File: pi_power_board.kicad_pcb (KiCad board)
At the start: 2 copper layers, 34.8 x 23.1 mm, 26 parts, among them J1 381camcon, J2 Conn_02x04_Odd_Even, Q1 SSM3K335R, Q2 SSM3K335R, Q3 DMG2305UX-7, U1 LM74610, U2 TPS2400, U3 DMMT5401

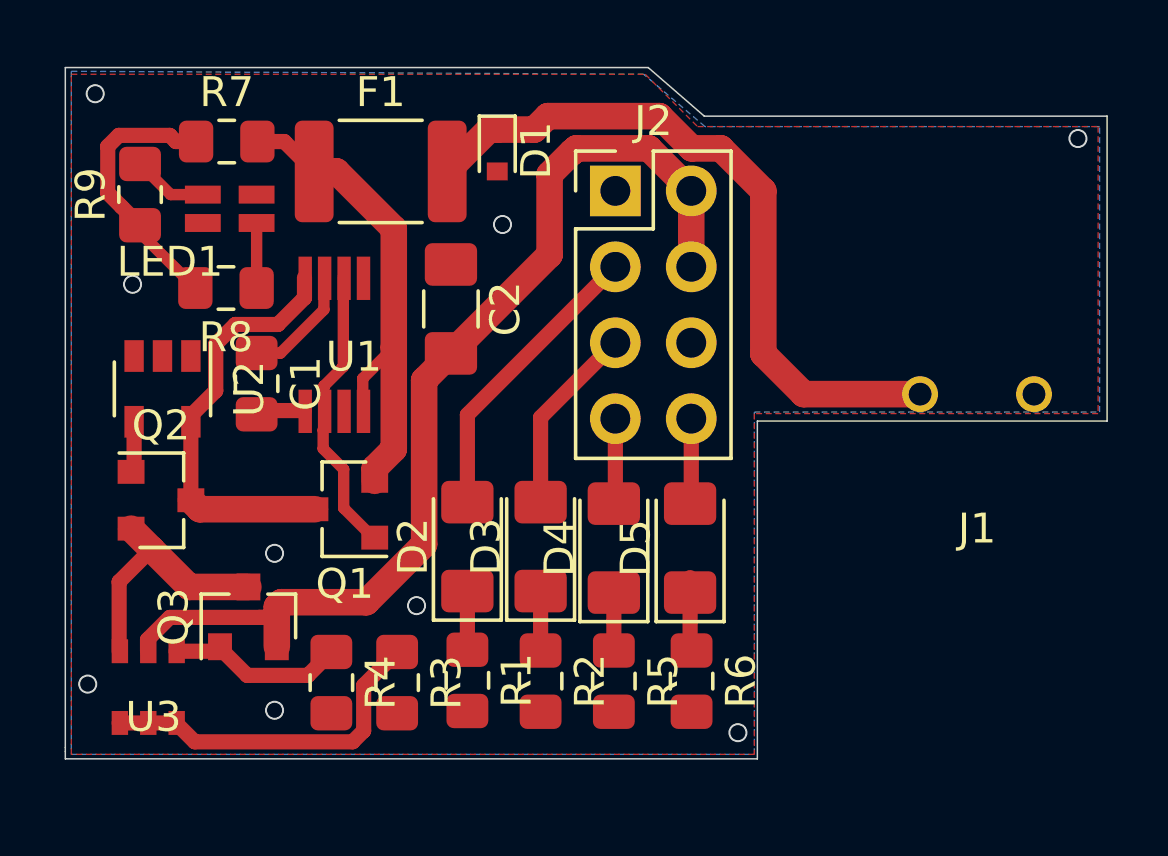
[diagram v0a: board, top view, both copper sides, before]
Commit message: Add files via upload
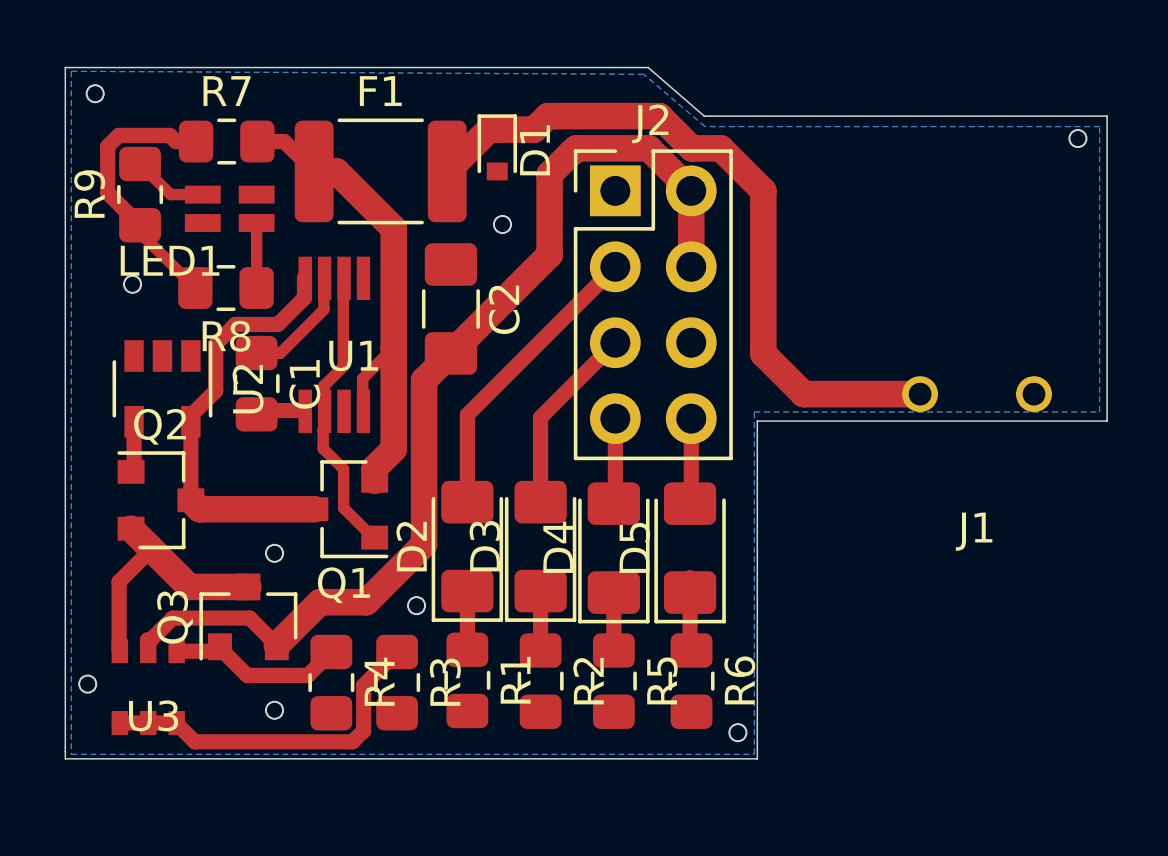
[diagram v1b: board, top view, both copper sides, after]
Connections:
- D1 pad 1: Net-(D1-Pad1) -> +VDC
- F1 pad 2: Net-(D1-Pad1) -> Net-(F1-Pad2)
- J1 pad 1: Net-(D1-Pad1) -> Net-(F1-Pad2)
- J2 pad 1: (no net) -> Net-(J2-Pad1)
- U1 pad 3: (no net) -> Net-(U1-Pad3)
- U1 pad 5: (no net) -> Net-(U1-Pad5)
- U2 pad 1: (no net) -> Net-(U2-Pad1)
- U2 pad 3: (no net) -> Net-(U2-Pad3)
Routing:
- removed copper zone on F.Cu, net GND
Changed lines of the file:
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@@
     (thickness 1.6)
     (drawings 15)
-    (tracks 130)
+    (tracks 129)
     (zones 0)
     (modules 26)
-    (nets 24)
+    (nets 30)
   )
   (page A4)
@@
   )
   (setup
-    (last_trace_width 0.254)
+    (last_trace_width 0.508)
     (user_trace_width 0.381)
     (user_trace_width 0.508)
@@
   (net 22 "Net-(LED1-Pad4)")
   (net 23 "Net-(R7-Pad1)")
+  (net 24 "Net-(F1-Pad2)")
+  (net 25 "Net-(J2-Pad1)")
+  (net 26 "Net-(U1-Pad3)")
+  (net 27 "Net-(U1-Pad5)")
+  (net 28 "Net-(U2-Pad1)")
+  (net 29 "Net-(U2-Pad3)")
   (net_class Default "This is the default net class."
     (clearance 0.127)
@@
     (add_net "Net-(D5-Pad1)")
     (add_net "Net-(D5-Pad2)")
+    (add_net "Net-(F1-Pad2)")
+    (add_net "Net-(J2-Pad1)")
     (add_net "Net-(LED1-Pad2)")
     (add_net "Net-(LED1-Pad4)")
@@
     (add_net "Net-(R3-Pad1)")
     (add_net "Net-(R7-Pad1)")
+    (add_net "Net-(U1-Pad3)")
+    (add_net "Net-(U1-Pad5)")
+    (add_net "Net-(U2-Pad1)")
+    (add_net "Net-(U2-Pad3)")
   )
   (module DMMT5401:DMMT5401 (layer F.Cu)
@@
       (net 4 GND))
     (pad 1 thru_hole circle (at -1.905 -4) (size 1.2 1.2) (drill 0.762) (layers *.Cu *.Mask)
-      (net 14 "Net-(D1-Pad1)"))
+      (net 24 "Net-(F1-Pad2)"))
   )
   (module APHBM2012:APHBM2012 (layer F.Cu)
@@
       (net 17 "Net-(Q1-Pad1)") (solder_mask_margin 0.05) (clearance 0.127))
     (pad 3 smd rect (at 0.3 2.1) (size 0.45 1.45) (drill (offset 0.025 0.025)) (layers F.Cu F.Adhes F.Paste F.SilkS F.Mask)
-      (solder_mask_margin 0.05) (clearance 0.127))
+      (net 26 "Net-(U1-Pad3)") (solder_mask_margin 0.05) (clearance 0.127))
     (pad 4 smd rect (at 0.95 2.1) (size 0.45 1.45) (drill (offset 0.025 0.025)) (layers F.Cu F.Adhes F.Paste F.SilkS F.Mask)
       (net 3 +VDC) (solder_mask_margin 0.05) (clearance 0.127))
@@
       (net 17 "Net-(Q1-Pad1)") (solder_mask_margin 0.05) (clearance 0.127))
     (pad 5 smd rect (at 0.95 -2.35) (size 0.45 1.45) (drill (offset 0.025 0.025)) (layers F.Cu F.Adhes F.Paste F.SilkS F.Mask)
-      (solder_mask_margin 0.05) (clearance 0.127))
+      (net 27 "Net-(U1-Pad5)") (solder_mask_margin 0.05) (clearance 0.127))
   )
   (module Package_TO_SOT_SMD:SOT-23 (layer F.Cu)
@@
     (fp_line (start 0.9 1.55) (end -0.9 1.55) (layer F.Fab) (width 0.1))
     (fp_line (start 0.9 -1.55) (end 0.9 1.55) (layer F.Fab) (width 0.1))
-    (pad 1 smd rect (at -1.1 -0.95 270) (size 1.06 0.65) (layers F.Cu F.Paste F.Mask))
+    (pad 1 smd rect (at -1.1 -0.95 270) (size 1.06 0.65) (layers F.Cu F.Paste F.Mask)
+      (net 28 "Net-(U2-Pad1)"))
     (pad 2 smd rect (at -1.1 0 270) (size 1.06 0.65) (layers F.Cu F.Paste F.Mask)
       (net 4 GND))
-    (pad 3 smd rect (at -1.1 0.95 270) (size 1.06 0.65) (layers F.Cu F.Paste F.Mask))
+    (pad 3 smd rect (at -1.1 0.95 270) (size 1.06 0.65) (layers F.Cu F.Paste F.Mask)
+      (net 29 "Net-(U2-Pad3)"))
     (pad 4 smd rect (at 1.1 0.95 270) (size 1.06 0.65) (layers F.Cu F.Paste F.Mask)
       (net 18 "Net-(Q2-Pad1)"))
@@
     (pad 2 thru_hole oval (at 2.54 0) (size 1.7 1.7) (drill 1) (layers *.Cu *.Mask)
       (net 13 +5V))
-    (pad 1 thru_hole rect (at 0 0) (size 1.7 1.7) (drill 1) (layers *.Cu *.Mask))
+    (pad 1 thru_hole rect (at 0 0) (size 1.7 1.7) (drill 1) (layers *.Cu *.Mask)
+      (net 25 "Net-(J2-Pad1)"))
     (model ${KISYS3DMOD}/Connector_PinHeader_2.54mm.3dshapes/PinHeader_2x04_P2.54mm_Vertical.wrl
       (at (xyz 0 0 0))
@@
     (fp_line (start -2.25 1.6) (end -2.25 -1.6) (layer F.Fab) (width 0.1))
     (pad 2 smd roundrect (at 2.225 0) (size 1.3 3.4) (layers F.Cu F.Paste F.Mask) (roundrect_rratio 0.192308)
-      (net 14 "Net-(D1-Pad1)"))
+      (net 24 "Net-(F1-Pad2)"))
     (pad 1 smd roundrect (at -2.225 0) (size 1.3 3.4) (layers F.Cu F.Paste F.Mask) (roundrect_rratio 0.192308)
       (net 3 +VDC))
@@
       (net 4 GND))
     (pad 1 smd rect (at -0.7 0 90) (size 0.6 0.7) (layers F.Cu F.Paste F.Mask)
-      (net 14 "Net-(D1-Pad1)"))
+      (net 3 +VDC))
     (model ${KISYS3DMOD}/Diode_SMD.3dshapes/D_SOD-523.wrl
       (at (xyz 0 0 0))
@@
   (segment (start 94.50349 131.575212) (end 94.50349 126.08401) (width 0.889) (layer F.Cu) (net 13))
   (segment (start 92.567702 133.511) (end 94.50349 131.575212) (width 0.889) (layer F.Cu) (net 13))
-  (segment (start 89.725 133.511) (end 92.567702 133.511) (width 0.889) (layer F.Cu) (net 13))
-  (segment (start 89.575 133.661) (end 89.725 133.511) (width 0.889) (layer F.Cu) (net 13))
-  (segment (start 89.575 135) (end 89.575 133.661) (width 0.889) (layer F.Cu) (net 13))
-  (segment (start 89.217001 134.018999) (end 88.981001 134.018999) (width 0.508) (layer F.Cu) (net 13))
-  (segment (start 89.575 133.661) (end 89.217001 134.018999) (width 0.508) (layer F.Cu) (net 13))
-  (segment (start 88.981001 134.018999) (end 89.118999 134.018999) (width 0.508) (layer F.Cu) (net 13))
   (segment (start 85.25 134.764198) (end 85.25 135.15) (width 0.508) (layer F.Cu) (net 13))
-  (segment (start 85.995199 134.018999) (end 85.25 134.764198) (width 0.508) (layer F.Cu) (net 13))
-  (segment (start 88.981001 134.018999) (end 85.995199 134.018999) (width 0.508) (layer F.Cu) (net 13))
+  (segment (start 91.014 133.511) (end 89.575 134.95) (width 0.889) (layer F.Cu) (net 13))
+  (segment (start 92.567702 133.511) (end 91.014 133.511) (width 0.889) (layer F.Cu) (net 13))
+  (segment (start 89.575 134.95) (end 89.575 135) (width 0.508) (layer F.Cu) (net 13))
+  (segment (start 88.667 134.042) (end 89.575 134.95) (width 0.508) (layer F.Cu) (net 13))
+  (segment (start 86.091573 134.042) (end 88.667 134.042) (width 0.508) (layer F.Cu) (net 13))
+  (segment (start 85.25 134.883573) (end 86.091573 134.042) (width 0.508) (layer F.Cu) (net 13))
+  (segment (start 85.25 135.15) (end 85.25 134.883573) (width 0.508) (layer F.Cu) (net 13))
   (segment (start 96.675 117.7) (end 96.95 117.7) (width 0.889) (layer F.Cu) (net 14))
   (segment (start 95.275 119.1) (end 96.675 117.7) (width 0.889) (layer F.Cu) (net 14))
@@
       )
     )
-  )
-  (zone (net 4) (net_name GND) (layer F.Cu) (hatch edge 0.508)
-    (connect_pads (clearance 0.127))
-    (min_thickness 0.254)
-    (fill yes (arc_segments 32) (thermal_gap 0.381) (thermal_bridge_width 0.381))
-    (polygon
-      (pts
-        (xy 82.7 115.85) (xy 101.9 115.85) (xy 103.65 117.6) (xy 117.05 117.6) (xy 117.05 127.2)
-        (xy 105.55 127.2) (xy 105.55 138.6) (xy 82.7 138.6)
-      )
-    )

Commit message: Add files via upload
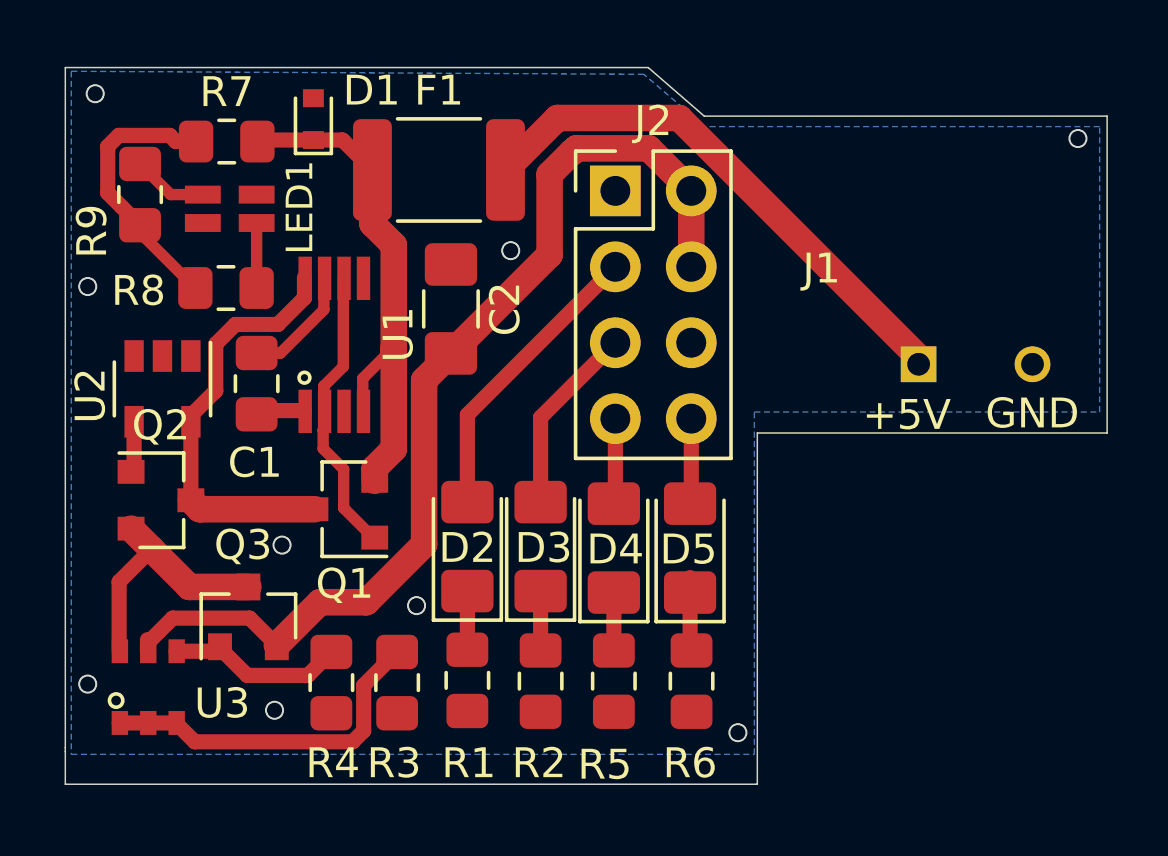
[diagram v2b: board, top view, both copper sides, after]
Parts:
- moved D1 6.24 mm to (90.8, 117.3), turned to 90 degrees
- moved F1 1.95 mm to (95.0, 119.0)
- moved J1 1.00 mm to (113.0, 129.6)
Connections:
- J2 pad 1: Net-(J2-Pad1) -> (no net)
- U1 pad 3: Net-(U1-Pad3) -> (no net)
- U1 pad 5: Net-(U1-Pad5) -> (no net)
- U2 pad 1: Net-(U2-Pad1) -> (no net)
- U2 pad 3: Net-(U2-Pad3) -> (no net)
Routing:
- net Net-(D1-Pad1): track 23.6 -> 0.00 mm
- net Net-(F1-Pad2): track 0.00 -> 18.1 mm
- net +VDC: track 17.5 -> 18.2 mm
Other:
- board size 34.8 x 23.1 mm -> 34.8 x 24 mm
- board text added: "+5V"
- board text added: "GND"

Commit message: Add files via upload
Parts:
- D1: value D5V0L1B2T-7 -> ESDA18-1K
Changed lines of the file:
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@@
   )
   (setup
-    (last_trace_width 0.889)
+    (last_trace_width 0.254)
     (user_trace_width 0.381)
     (user_trace_width 0.508)
@@
       (effects (font (size 1 1) (thickness 0.15)))
     )
-    (fp_text value D5V0L1B2T-7 (at 0 1.4 90) (layer F.Fab)
-      (effects (font (size 1 1) (thickness 0.15)))
-    )
+    (fp_text value ESDA18-1K (at 0 1.4 90) (layer F.Fab)
+      (effects (font (size 1 1) (thickness 0.15)))
+    )
